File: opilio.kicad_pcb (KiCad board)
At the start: 4 copper layers, 80 x 40 mm, 89 parts, among them J1 Screw_Terminal_01x02, J2 USB_B_Micro, J3 Conn_01x02_Male, J4 Conn_01x02_Male, J5 Conn_01x02_Male, Q1 PMV25ENEAR, Q2 AO3401A, U1 EUP3458, U2 STM32F103C8T6, Y1 YSX531SL 8MHz, Y2 YST310S 32.768KHz

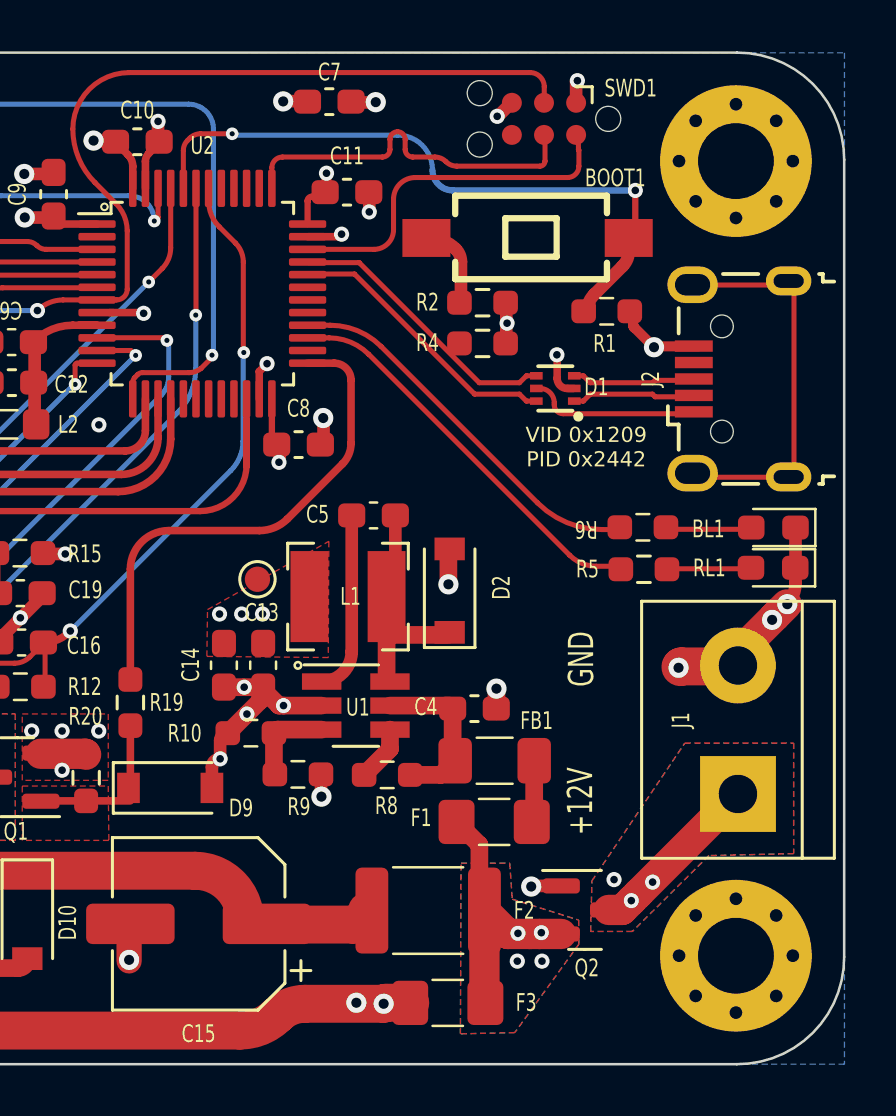
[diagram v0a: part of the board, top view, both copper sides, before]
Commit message: cleanup and annotate schema
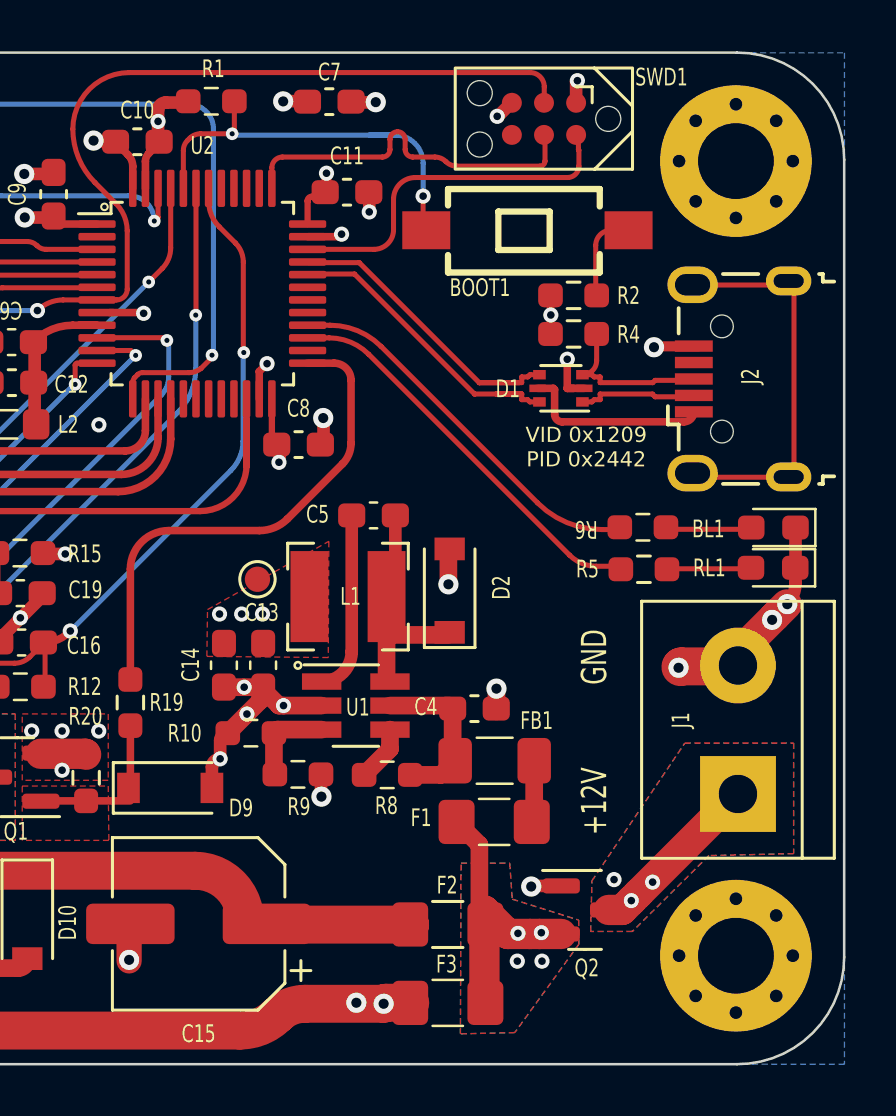
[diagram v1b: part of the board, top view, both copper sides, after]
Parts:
- D1: footprint easyeda2kicad:SOT-666-6_L1.6-W1.2-P0.50-LS1.6-BL -> Package_TO_SOT_SMD:SOT-666
- F2: value 3A -> 2A; footprint Fuse:Fuse_1812_4532Metric_Pad1.30x3.40mm_HandSolder -> Fuse:Fuse_1206_3216Metric_Pad1.42x1.75mm_HandSolder
- R20: value 10K -> 7k5
- moved R1 17.7 mm to (155.0, 101.9), turned to 180 degrees
- moved R4 3.62 mm to (169.3, 111.1), turned to 0 degrees
- moved R2 3.61 mm to (169.3, 109.6), turned to 0 degrees
- moved F2 0.95 mm to (164.3, 134.5)
- moved BOOT1 0.31 mm to (167.5, 107.0), turned to 0 degrees
- moved D1 0.22 mm to (168.8, 113.3), turned to 180 degrees
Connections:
- R4 pad 2: USB_D+ -> USB_CON_D+
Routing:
- net BOOT0: track 25.9 -> 16.9 mm
- net USB_D-: track 11.1 -> 13.3 mm
- net USB_D+: track 11.1 -> 13.0 mm
- net USB_CON_D+: track 4.49 -> 6.21 mm
- net +12VF(P): track 26.3 -> 27.8 mm
- net +5V: track 6.80 -> 7.54 mm
- net +3.3V: track 25.8 -> 26.3 mm
